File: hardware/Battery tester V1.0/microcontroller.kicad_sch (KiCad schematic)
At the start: 17 parts, among them IC4 PIC18F67J50, J1 USB_B, J2 ICP

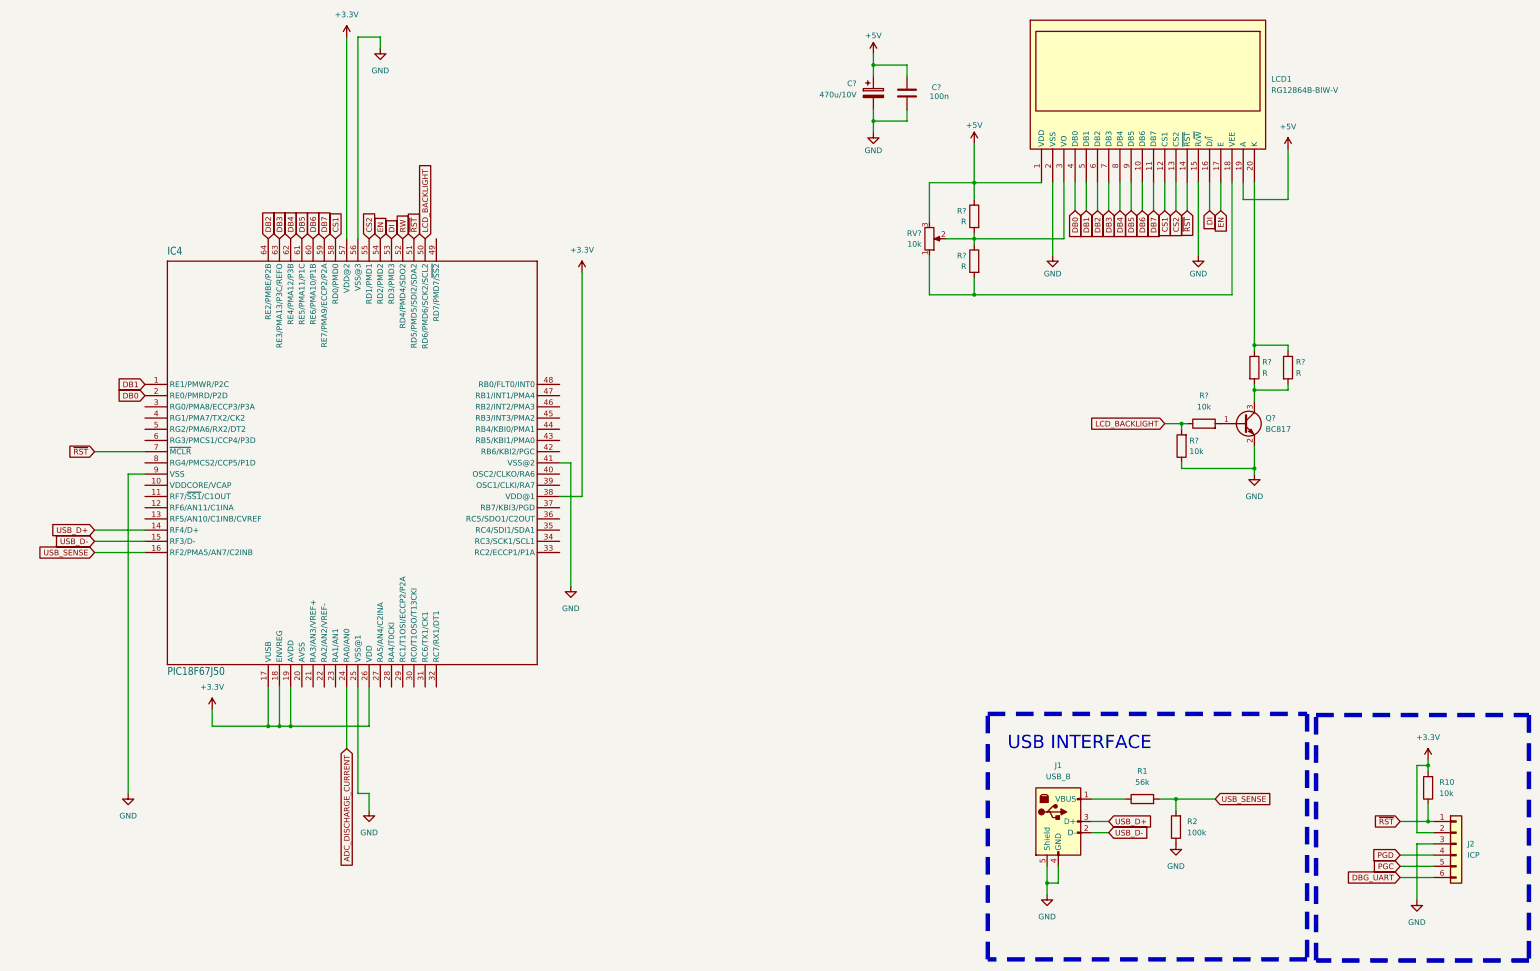
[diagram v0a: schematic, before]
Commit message: update man pcb, cleanup
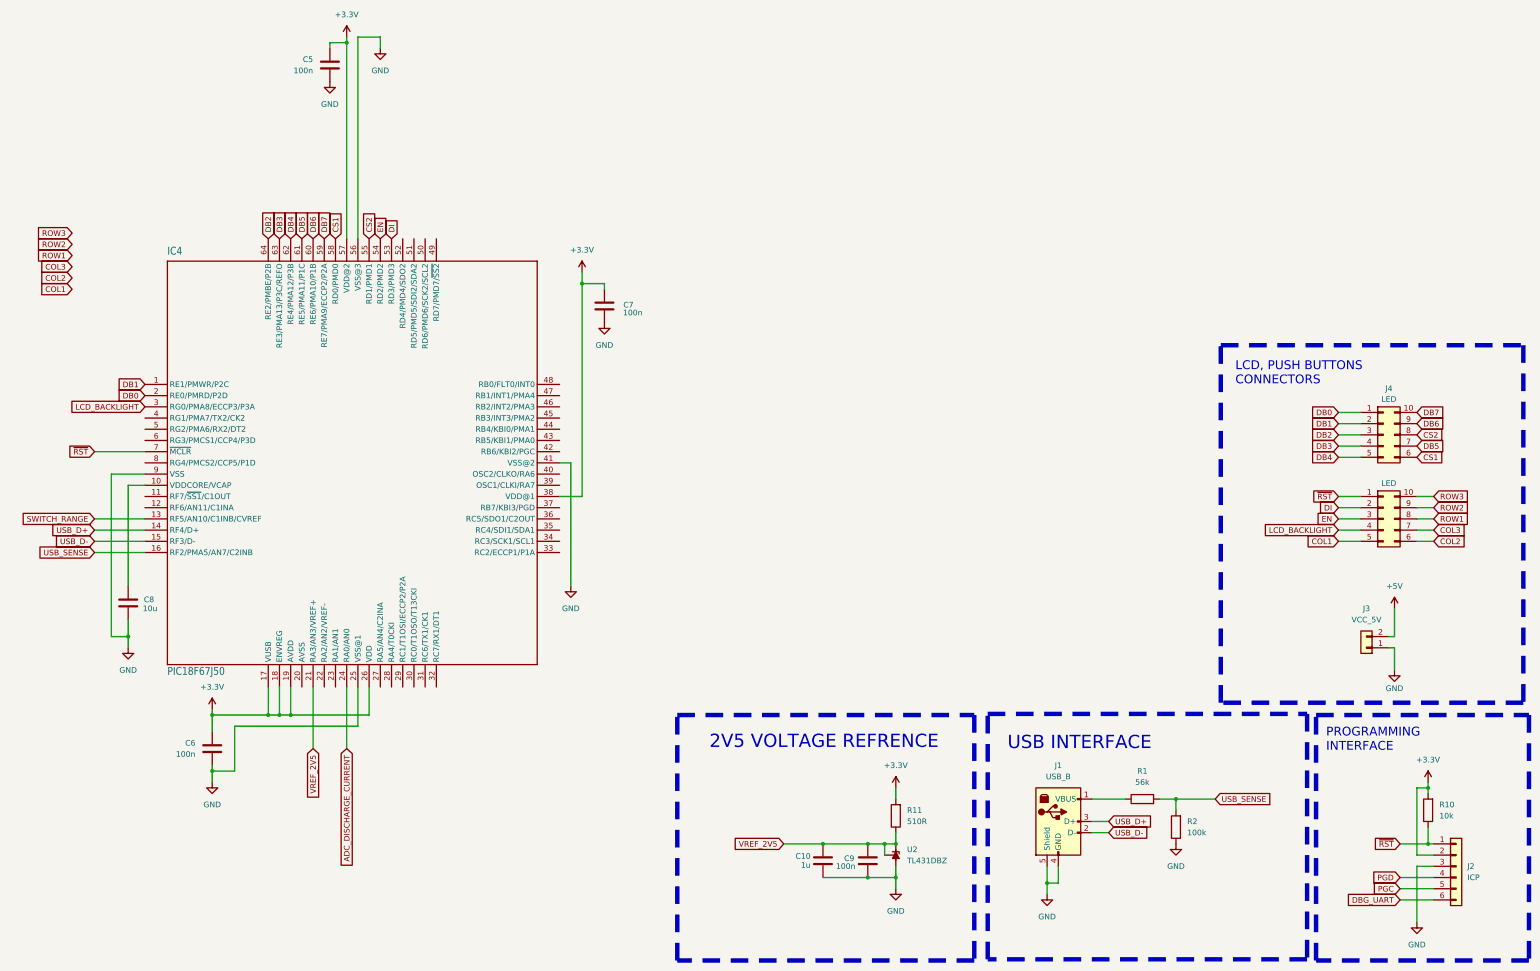
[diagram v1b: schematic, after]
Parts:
- removed C?: 470u/10V, Capacitor_THT:CP_Radial_D8.0mm_P3.80mm, symbol Device:C_Polarized
- removed C?: 100n, Capacitor_SMD:C_0805_2012Metric_Pad1.18x1.45mm_HandSolder, symbol Device:C
- removed LCD1: RG12864B-BIW-V, symbol My-Lib:RG12864B-BIW-V
- removed Q?: BC817, Package_TO_SOT_SMD:SOT-23, symbol Transistor_BJT:BC817
- removed R? (x2): 10k, Resistor_SMD:R_0805_2012Metric, symbol Device:R
- removed R? (x2): R, Resistor_SMD:R_1206_3216Metric, symbol Device:R
- removed R? (x2): R, Resistor_SMD:R_0805_2012Metric_Pad1.20x1.40mm_HandSolder, symbol Device:R
- removed RV?: 10k, Potentiometer_THT:Potentiometer_ACP_CA9-V10_Vertical_Hole, symbol Device:R_Potentiometer
- added C10: 1u, Capacitor_SMD:C_0805_2012Metric_Pad1.18x1.45mm_HandSolder, symbol Device:C
- added C5, C6, C7, C9: 100n, Capacitor_SMD:C_0805_2012Metric_Pad1.18x1.45mm_HandSolder, symbol Device:C
- added C8: 10u, Capacitor_SMD:C_1206_3216Metric_Pad1.33x1.80mm_HandSolder, symbol Device:C
- added J3: VCC_5V, Connector_JST:JST_XA_B02B-XASK-1_1x02_P2.50mm_Vertical, symbol Connector_Generic:Conn_01x02
- added J3, J4: LED, Connector_IDC:IDC-Header_2x05_P2.54mm_Vertical, symbol Connector_Generic:Conn_02x05_Counter_Clockwise
- added R11: 510R, symbol Device:R
- added U2: TL431DBZ, Package_TO_SOT_SMD:SOT-23, symbol Reference_Voltage:TL431DBZ
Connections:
- net +3.3V: now also C5.1, C6.1, C7.1, R11.2
- net +5V: now also J3.2 (Pin_2)
- net CS1: now also J4.6 (Pin_6)
- net CS2: now also J4.8 (Pin_8)
- net DB0: now also J4.1 (Pin_1)
- net DB1: now also J4.2 (Pin_2)
- net DB2: now also J4.3 (Pin_3)
- net DB3: now also J4.4 (Pin_4)
- net DB4: now also J4.5 (Pin_5)
- net DB5: now also J4.7 (Pin_7)
- net DB6: now also J4.9 (Pin_9)
- net DB7: now also J4.10 (Pin_10)
- net DI: now also J3.2 (Pin_2)
- net EN: now also J3.3 (Pin_3)
- net GND: now also C10.2, C5.2, C6.2, C7.2, C8.2, C9.2, J3.1 (Pin_1), U2.3 (A)
- net LCD_BACKLIGHT: now also IC4.3 (RG0/PMA8/ECCP3/P3A), J3.4 (Pin_4); no longer IC4.50 (RD6/PMD6/SCK2/SCL2)
- net ~{RST}: now also J3.1 (Pin_1); no longer IC4.51 (RD5/PMD5/SDI2/SDA2)
- net at IC4.10 (VDDCORE/VCAP): now also C8.1
- net SWITCH_RANGE: now reaches IC4.13 (RF5/AN10/C1INB/CVREF)
- net VREF_2V5: now reaches IC4.21 (RA3/AN3/VREF+)
- net VREF_2V5: now also C10.1, C9.1, R11.1, U2.1 (K), U2.2 (REF)
- net RW: no longer names the net of IC4.52 (RD4/PMD4/SDO2)
- new net COL1: J3.5 (Pin_5)
- new net COL2: J3.6 (Pin_6)
- new net COL3: J3.7 (Pin_7)
- new net ROW1: J3.8 (Pin_8)
- new net ROW2: J3.9 (Pin_9)
- new net ROW3: J3.10 (Pin_10)
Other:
- note added: "2V5 VOLTAGE REFRENCE"
- note added: "LCD, PUSH BUTTONS CONNECTORS"
- note added: "PROGRAMMING INTERFACE"
- moved on the sheet: J2, R10
